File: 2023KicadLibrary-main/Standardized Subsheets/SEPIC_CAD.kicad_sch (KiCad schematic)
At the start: 25 parts, among them IC1 LM5155DSSR, Q1 CSD18537NQ5A

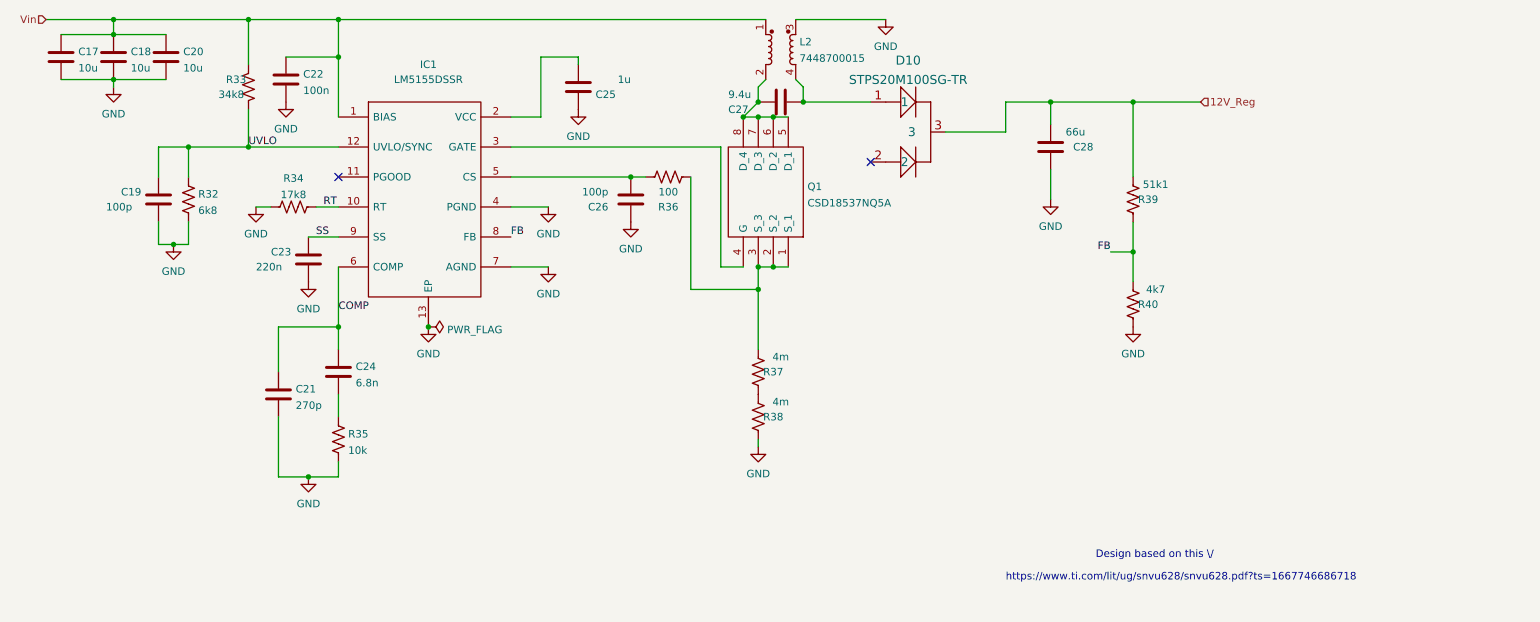
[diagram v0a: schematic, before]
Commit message: new HUD PCB
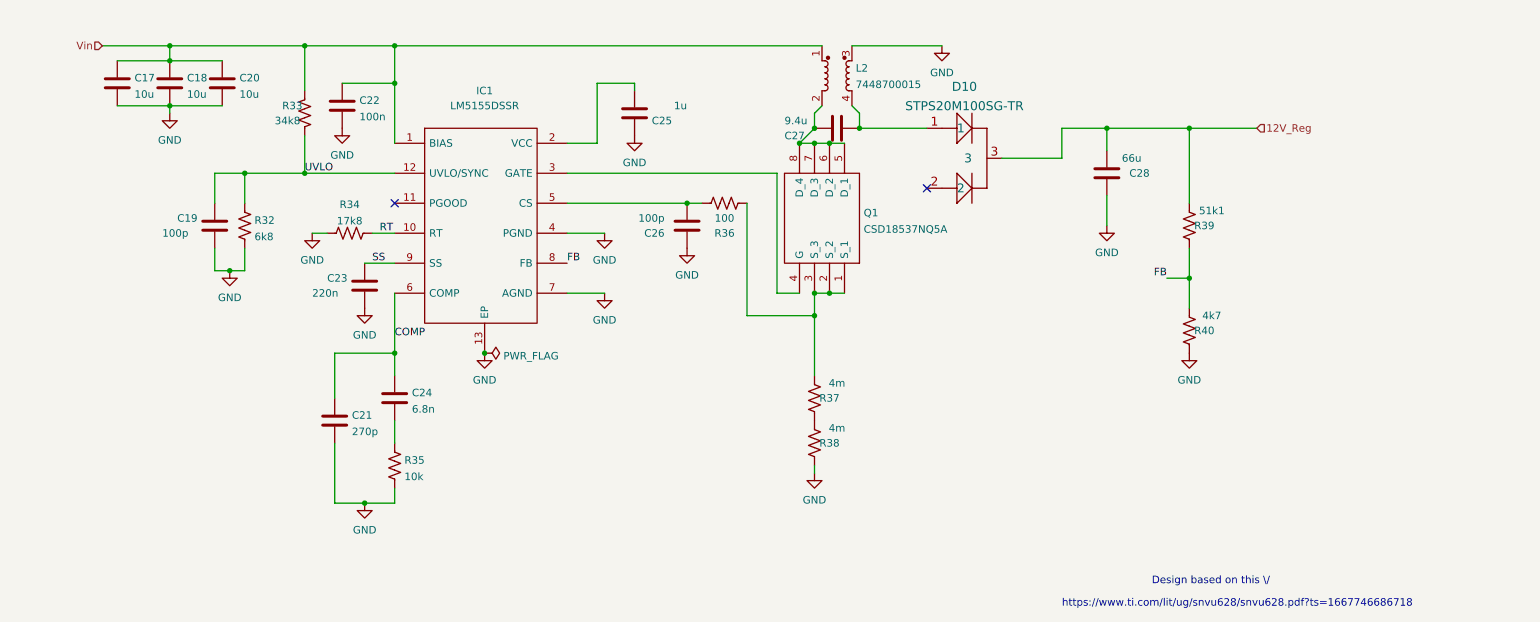
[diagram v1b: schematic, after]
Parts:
- C17, C18, C19, C20, C21, C22, C23, C24, C25, C26, C27, C28: footprint (none) -> Capacitor_SMD:C_0603_1608Metric
- D10: footprint D2PAK_STM -> Global Libraries_2:STPS20M100SG-TR
- L2: footprint (none) -> Inductor Thing:WE-DD_12XX_CROSSED12
- R32, R33, R34, R35, R36, R37, R38, R39, R40: footprint (none) -> Resistor_SMD:R_0603_1608Metric
